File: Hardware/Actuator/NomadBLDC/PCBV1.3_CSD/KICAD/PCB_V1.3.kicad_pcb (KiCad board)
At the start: 4 copper layers, 42.7 x 37.2 mm, 66 parts, among them J1 Conn_01x03, J2 USB_B_Micro, U1 CSD88599Q5DC, U3 CSD88599Q5DC, U4 CSD88599Q5DC

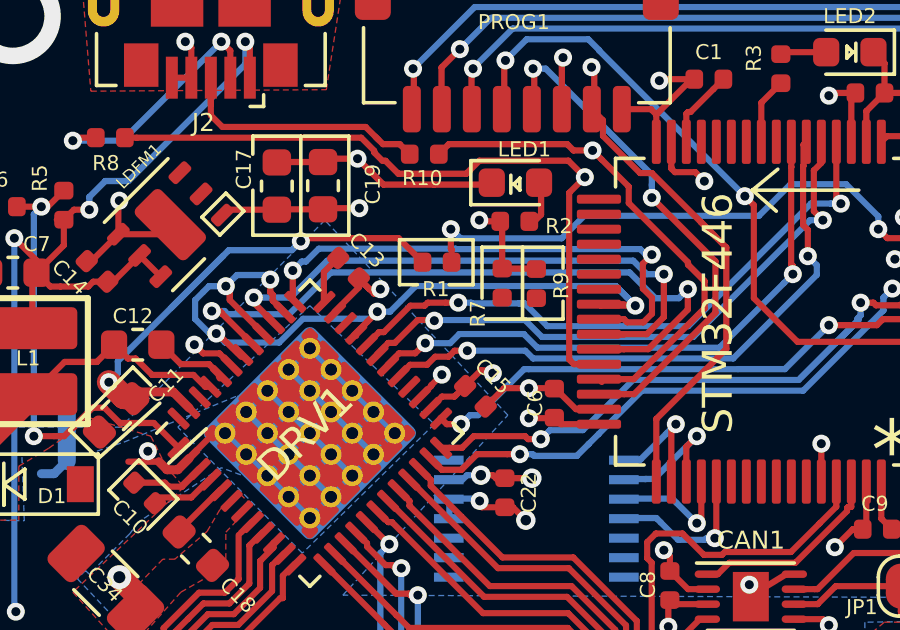
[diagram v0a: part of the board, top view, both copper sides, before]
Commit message: updated some files
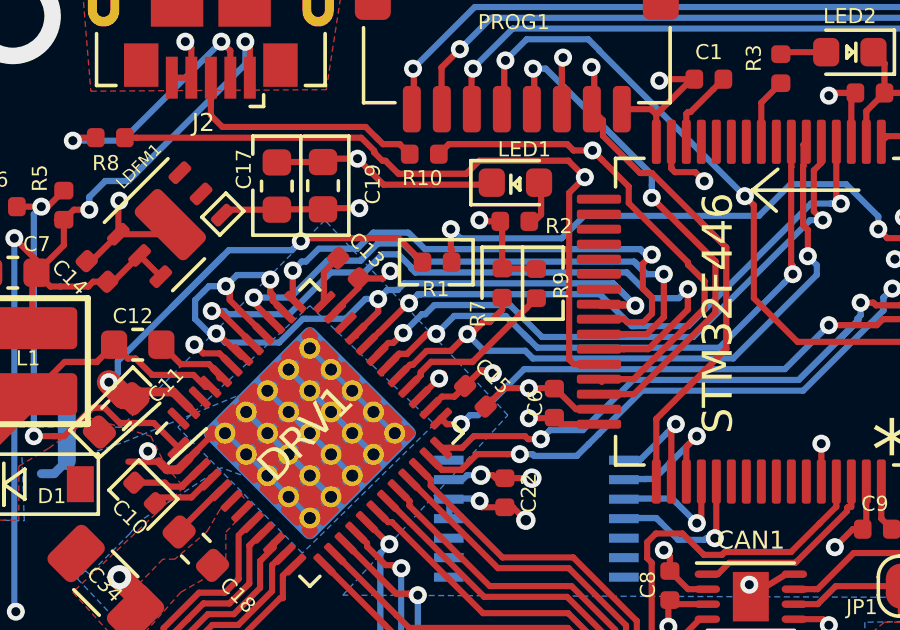
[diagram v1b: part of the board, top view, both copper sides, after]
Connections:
- R7 pad 2: Net-(R7-Pad2) -> /SPI-MISO
- R9 pad 1: Net-(R9-Pad1) -> /FAULT
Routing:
- net /FAULT: track 0.00 -> 5.52 mm
- net /SPI-MISO: track 20.2 -> 22.9 mm
- net /SPI-MOSI: track 19.6 -> 20.9 mm
- net ENABLE: track 28.8 -> 29.8 mm
- net PWMB: track 20.5 -> 21.3 mm
- net /SPI-SCK: track 20.0 -> 20.7 mm
- net PWMA: track 24.0 -> 24.5 mm
- net PWMC: track 17.6 -> 18.1 mm
